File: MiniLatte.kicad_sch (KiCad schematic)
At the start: 5 parts, among them SW1 SW_Push, SW2 SW_Push

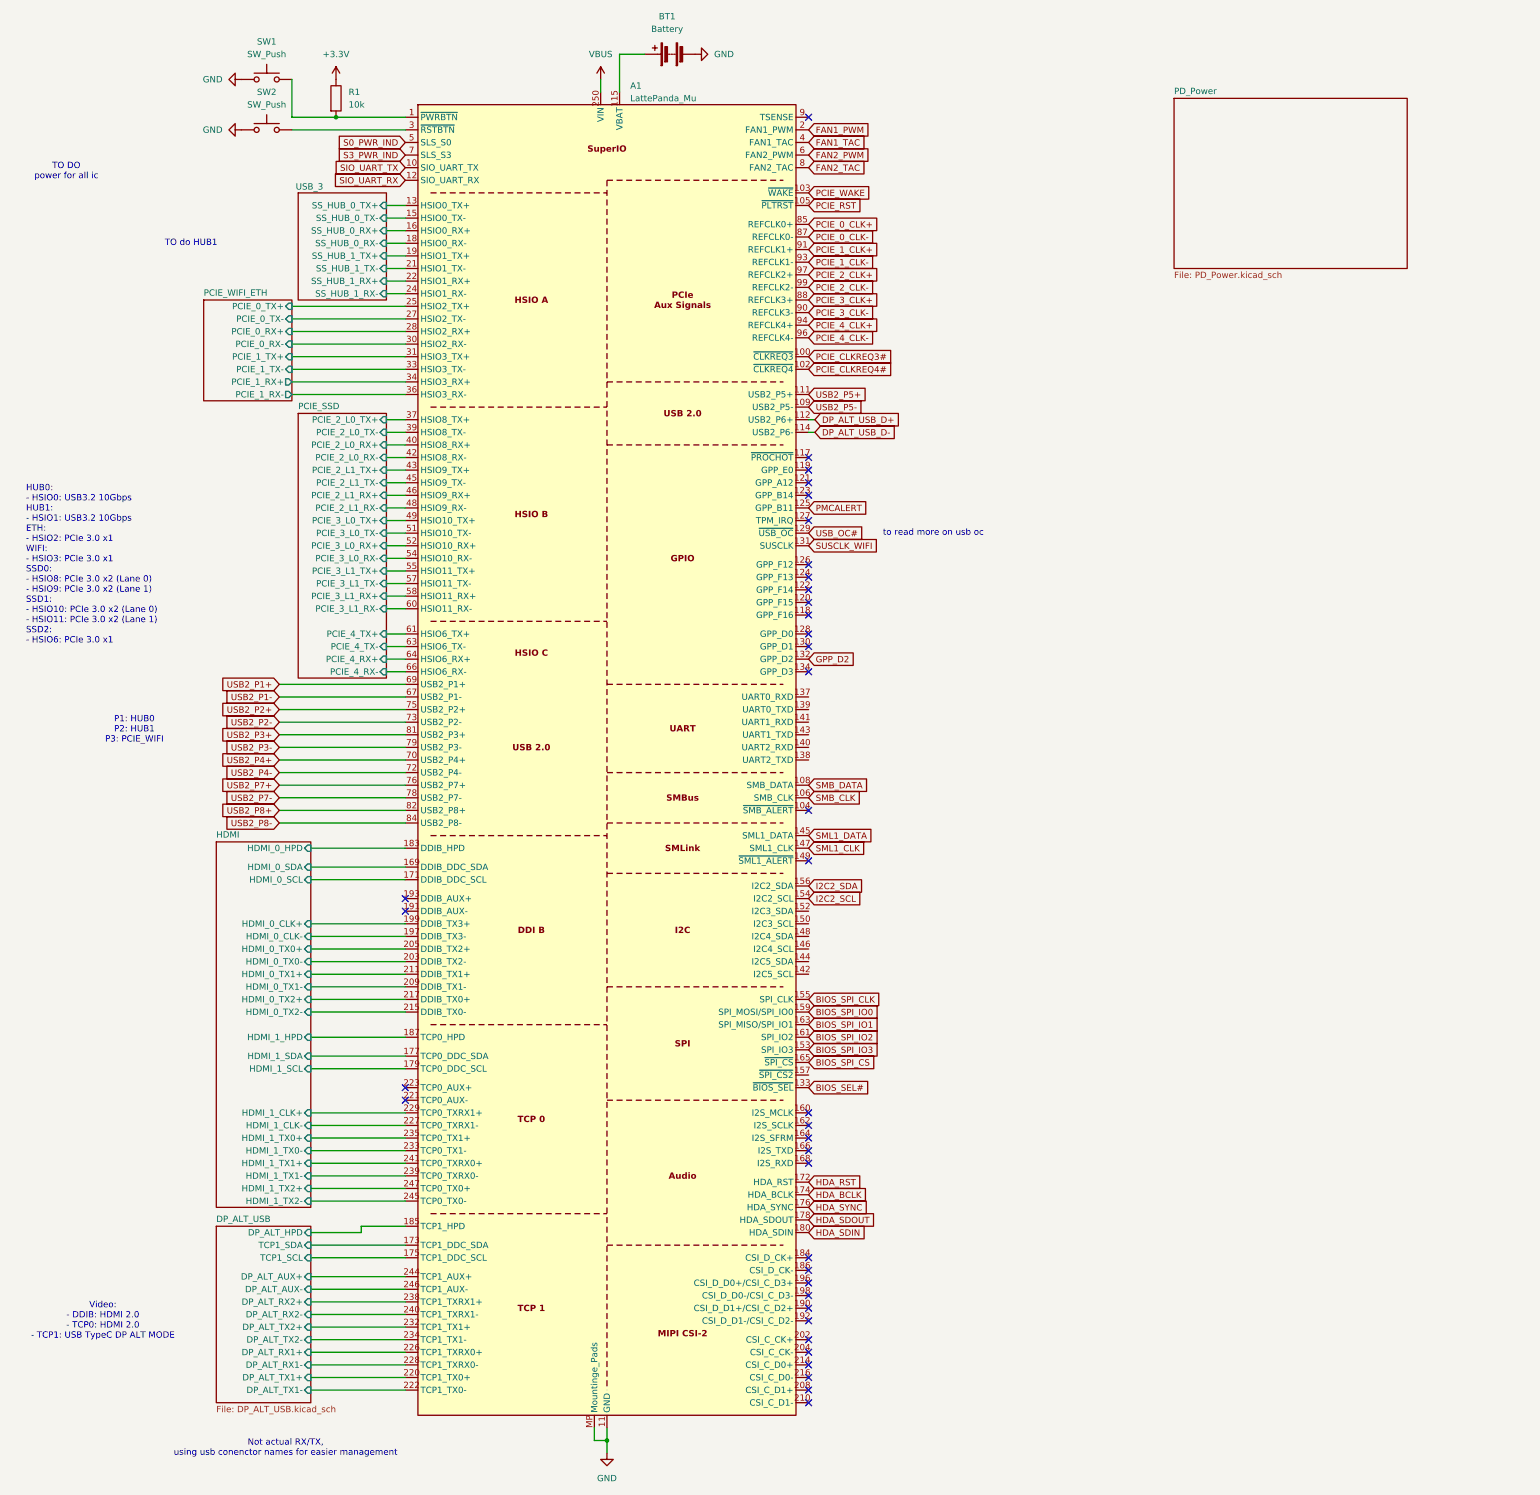
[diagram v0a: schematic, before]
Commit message: .
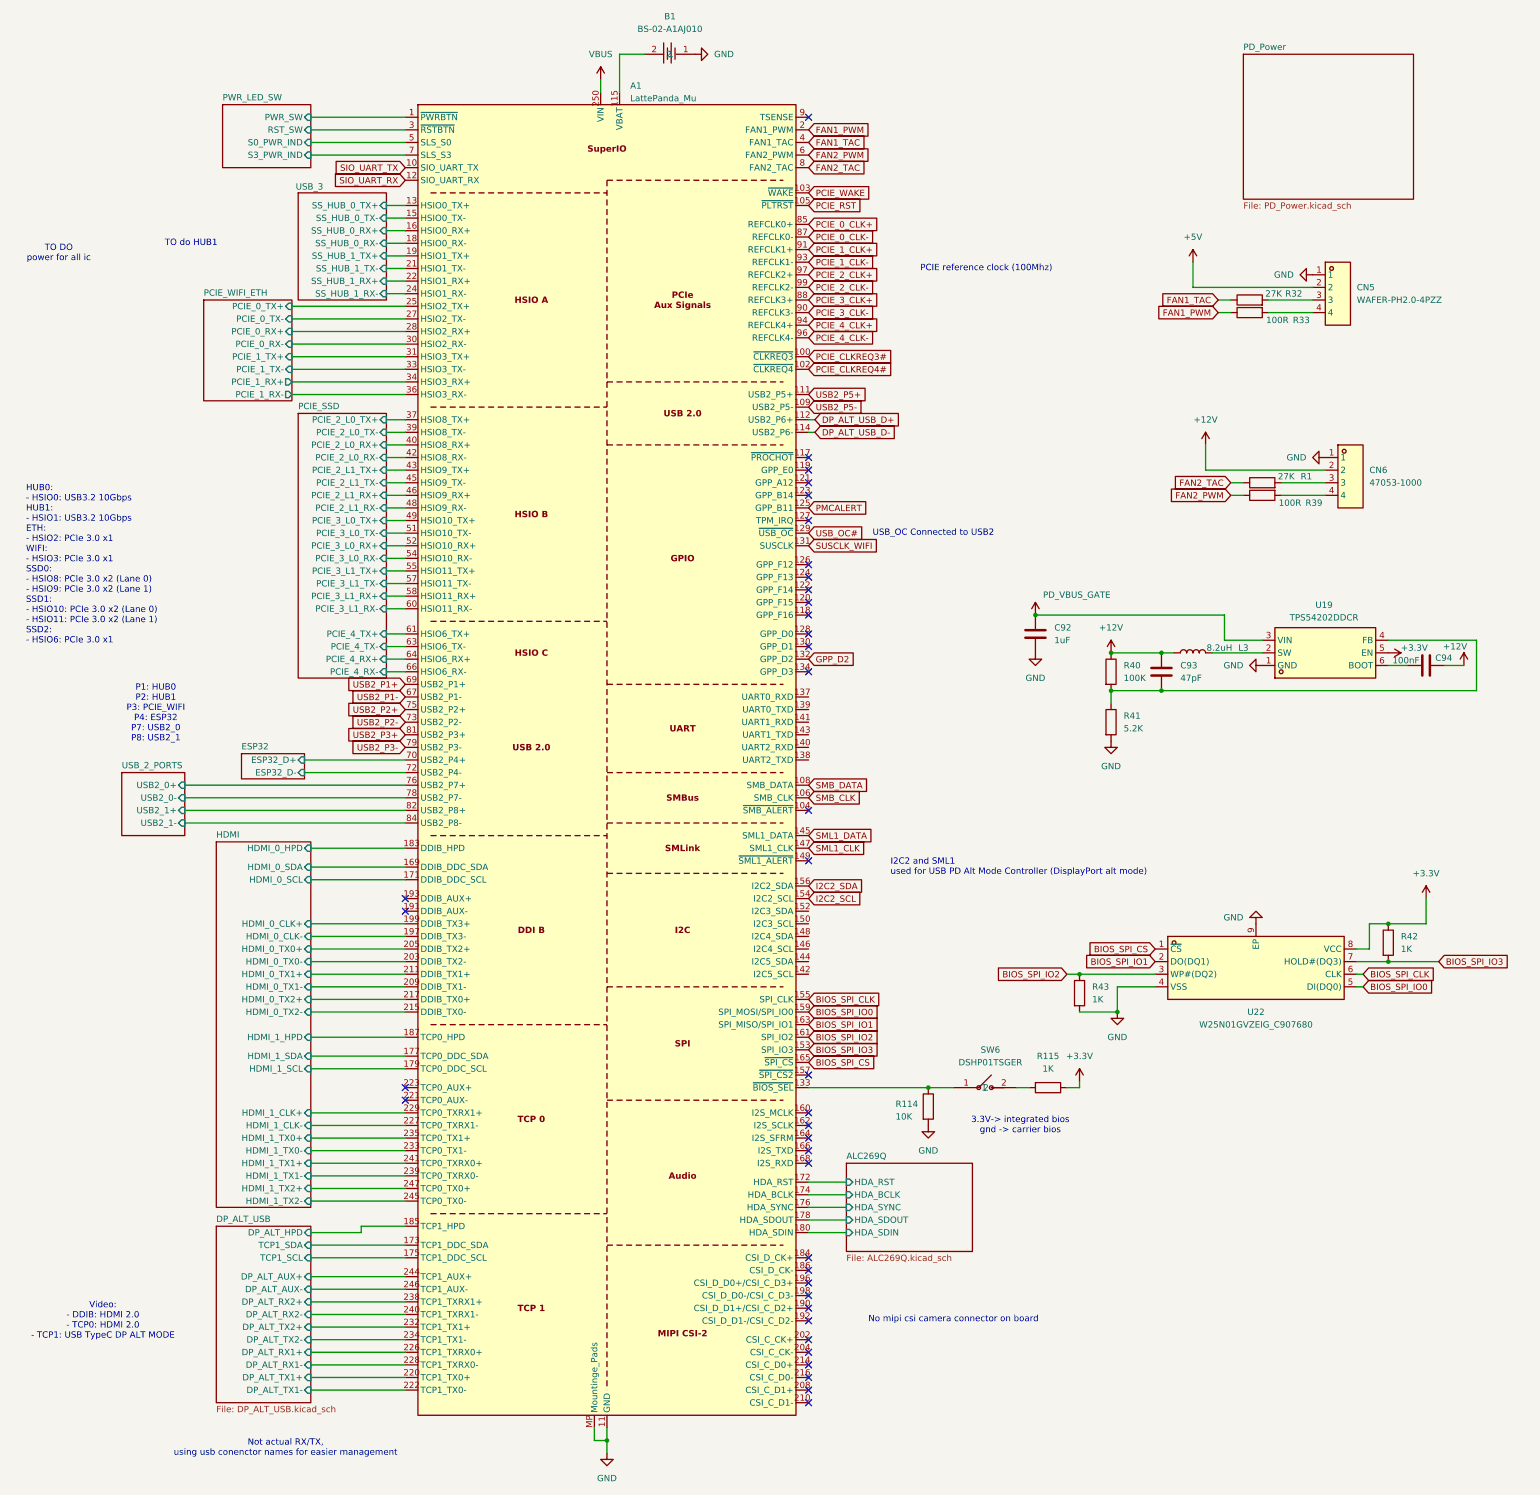
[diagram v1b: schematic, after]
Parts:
- removed BT1: Battery, symbol Device:Battery
- removed SW1, SW2: SW_Push, symbol Switch:SW_Push
- added B1: BS-02-A1AJ010, easyeda2kicad:BAT-TH_BS-02-A1AJ010, symbol da:BS-02-A1AJ010
- added C92: 1uF, Capacitor_SMD:C_0603_1608Metric, symbol Device:C
- added C93: 47pF, Capacitor_SMD:C_0402_1005Metric, symbol Device:C
- added C94: 100nF, Capacitor_SMD:C_0402_1005Metric, symbol Device:C
- added CN5: WAFER-PH2.0-4PZZ, easyeda2kicad:CONN-TH_4P-P2.00_FWF20001-S04S22W5B, symbol da:WAFER-PH2.0-4PZZ
- added CN6: 47053-1000, easyeda2kicad:CONN-TH_47053-1000, symbol da:47053-1000
- added L3: 8.2uH, Inductor_SMD:L_Changjiang_FXL0420, symbol Device:L
- added R114: 10K, Resistor_SMD:R_0402_1005Metric, symbol Device:R
- added R115, R42, R43: 1K, Resistor_SMD:R_0402_1005Metric, symbol Device:R
- added R32: 27K, Resistor_SMD:R_0402_1005Metric, symbol Device:R
- added R33, R39: 100R, Resistor_SMD:R_0402_1005Metric, symbol Device:R
- added R40: 100K, Resistor_SMD:R_0402_1005Metric, symbol Device:R
- added R41: 5.2K, Resistor_SMD:R_0402_1005Metric, symbol Device:R
- added SW6: DSHP01TSGER, easyeda2kicad:SW-SMD_DSHP01TSGER, symbol da:DSHP01TSGER
- added U19: TPS54202DDCR, easyeda2kicad:SOT-23-6_L2.9-W1.6-P0.95-LS2.8-BL, symbol da:TPS54202DDCR
- added U22: W25N01GVZEIG_C907680, easyeda2kicad:WSON-8_L8.0-W6.10-P1.27-BL-EP, symbol da:W25N01GVZEIG_C907680
- R1: value 10k -> 27K
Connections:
- net +3.3V: now also R115.1, R42.1, U19.5 (EN), U22.8 (VCC); no longer R1.1
- net BIOS_SPI_CLK: now also U22.6 (CLK)
- net BIOS_SPI_CS: now also U22.1 (~{CS})
- net BIOS_SPI_IO0: now also U22.5 (DI(DQ0))
- net BIOS_SPI_IO1: now also U22.2 (DO(DQ1))
- net BIOS_SPI_IO2: now also R43.1, U22.3 (WP#(DQ2))
- net BIOS_SPI_IO3: now also R42.2, U22.7 (HOLD#(DQ3))
- net FAN1_PWM: now also R33.1
- net FAN1_TAC: now also R32.1
- net FAN2_PWM: now also R39.1
- net FAN2_TAC: now also R1.1
- net GND: now also B1.1, C92.2, CN5.1, CN6.1, R114.2, R41.2, R43.2, U19.1 (GND), U22.4 (VSS), U22.9 (EP)
- net PWR_LED_SW/RST_SW: now reaches A1.3 (~{RSTBTN})
- net at A1.115 (VBAT): now also B1.2
- net at R1.2: now also CN6.3; no longer A1.1 (~{PWRBTN})
- net BIOS_SEL#: no longer names the net of A1.133 (~{BIOS_SEL})
- net BIOS_SEL#: now also R114.1, SW6.1
- net HDA_BCLK renamed ALC269Q/HDA_BCLK
- net HDA_RST renamed ALC269Q/HDA_RST
- net HDA_SDIN renamed ALC269Q/HDA_SDIN
- net HDA_SDOUT renamed ALC269Q/HDA_SDOUT
- net HDA_SYNC renamed ALC269Q/HDA_SYNC
- net S0_PWR_IND renamed PWR_LED_SW/S0_PWR_IND
- net S3_PWR_IND renamed PWR_LED_SW/S3_PWR_IND
- net USB2_P4+ renamed ESP32/ESP32_D+
- net USB2_P4- renamed ESP32/ESP32_D-
- net USB2_P7+ renamed USB_2_PORTS/USB2_0+
- net USB2_P7- renamed USB_2_PORTS/USB2_0-
- net USB2_P8+ renamed USB_2_PORTS/USB2_1+
- net USB2_P8- renamed USB_2_PORTS/USB2_1-
- new net: L3.2, U19.2 (SW)
- new net: C93.2, R40.2, R41.1, U19.4 (FB)
- new net: C94.1, U19.6 (BOOT)
- new net: CN6.4, R39.2
- new net: R115.2, SW6.2
- new net: CN5.3, R32.2
- new net: CN5.4, R33.2
- new net +12V: C93.1, C94.2, CN6.2, L3.1, R40.1
- new net +5V: CN5.2
- new net PD_VBUS_GATE: C92.1, U19.3 (VIN)
- new net PWR_LED_SW/PWR_SW: A1.1 (~{PWRBTN})
- no-connect marks 37 -> 38
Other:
- added sheet ALC269Q (ALC269Q.kicad_sch)
- added sheet ESP32 (ESP32.kicad_sch)
- added sheet PWR_LED_SW (PWR_LED.kicad_sch)
- added sheet USB_2_PORTS (USB_2_PORTS.kicad_sch)
- note added: "3.3V-> integrated bios gnd -> carrier bios"
- note added: "I2C2 and SML1 used for USB PD Alt Mode Controller (DisplayPort alt mode)"
- note added: "No mipi csi camera connector on board"
- note added: "P1: HUB0 P2: HUB1 P3: PCIE_WIFI P4: ESP32 P7: USB2_0 P8: USB2_1"
- note added: "PCIE reference clock (100Mhz)"
- note added: "USB_OC Connected to USB2"
- note removed: "P1: HUB0 P2: HUB1 P3: PCIE_WIFI"
- note removed: "to read more on usb oc"
